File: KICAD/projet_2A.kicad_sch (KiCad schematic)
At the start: 3 parts, among them IC3 PCM1808PW, IC4 PCM5102AQPWRQ1, U1 FSC-BT1026E

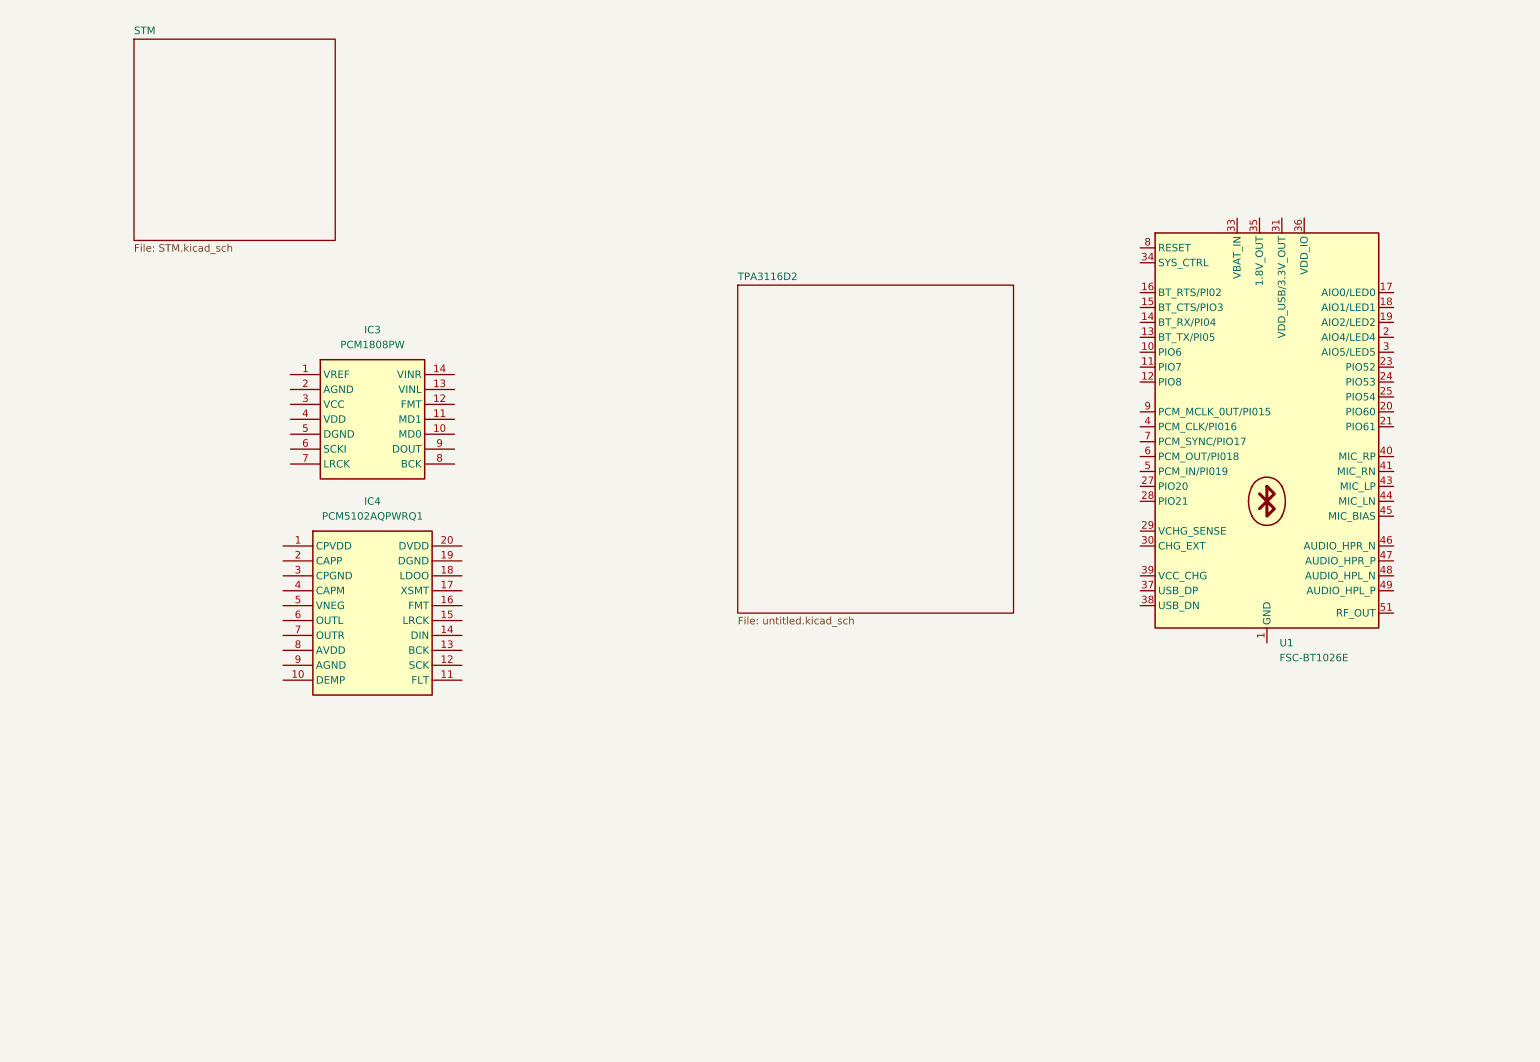
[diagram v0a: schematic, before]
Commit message: BT + PCM1808
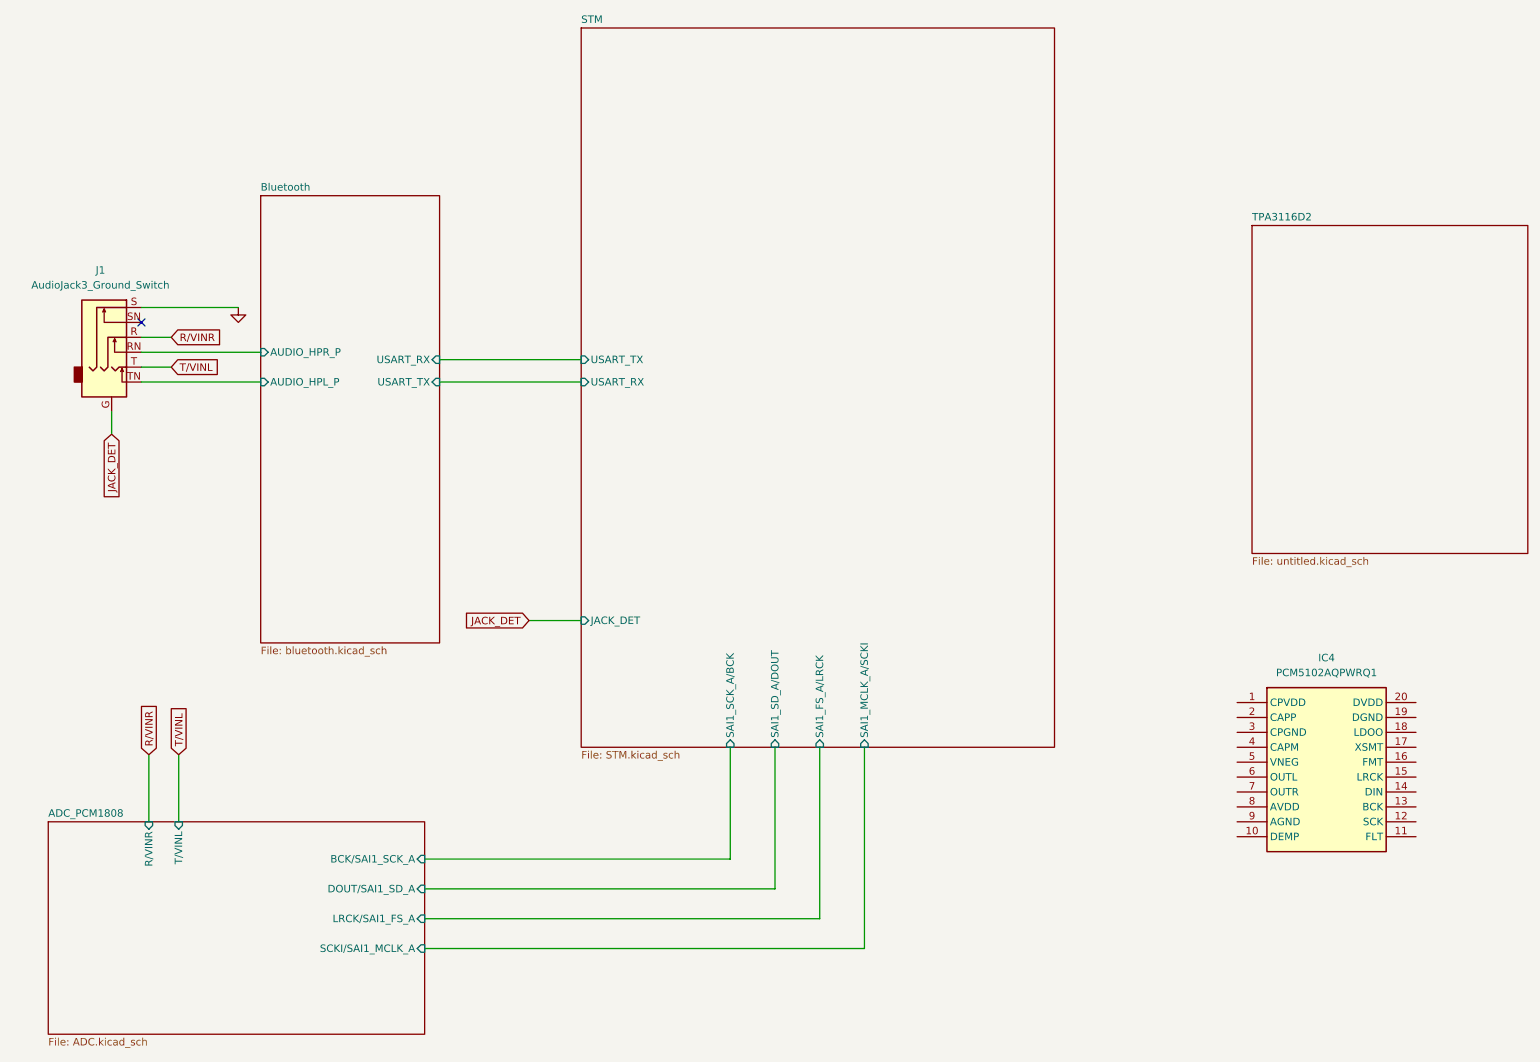
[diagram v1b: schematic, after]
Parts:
- removed IC3: PCM1808PW, Package_SO:TSSOP-14_4.4x5mm_P0.65mm, symbol PCM1808PW:PCM1808PW
- removed U1: FSC-BT1026E, Bluetooth:FSC-BT1026x, symbol Bluetooth_FSC_BT1026x:FSC-BT1026x
- added J1: AudioJack3_Ground_Switch, symbol Connector_Audio:AudioJack3_Ground_Switch
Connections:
- new net Bluetooth/AUDIO_HPL_P: J1.TN
- new net Bluetooth/AUDIO_HPR_P: J1.RN
- new net GND: J1.S
- new net JACK_DET: J1.G
- new net R/VINR: J1.R
- new net T/VINL: J1.T
- no-connect marks 0 -> 1
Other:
- added sheet ADC_PCM1808 (ADC.kicad_sch)
- added sheet Bluetooth (bluetooth.kicad_sch)
- sheet STM ports: added JACK_DET, SAI1_FS_A/LRCK, SAI1_MCLK_A/SCKI, SAI1_SCK_A/BCK, SAI1_SD_A/DOUT, USART_RX, USART_TX; removed none
- moved on the sheet: IC4
